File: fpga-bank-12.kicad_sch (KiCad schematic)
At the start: 1 part, among them U4 XC7K160T-FFG676

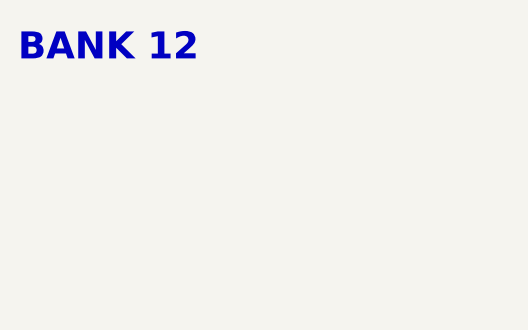
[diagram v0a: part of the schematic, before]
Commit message: Finish schematic cleanup
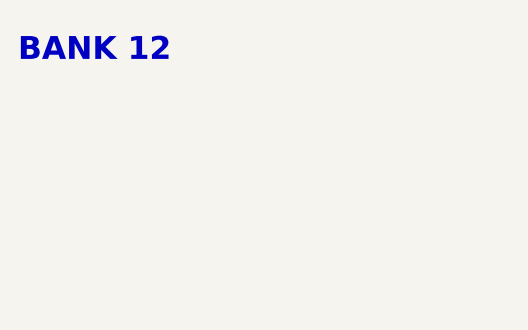
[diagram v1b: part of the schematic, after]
